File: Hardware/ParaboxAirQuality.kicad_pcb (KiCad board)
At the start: 2 copper layers, 25 parts, among them J1 USB_B_Mini, J2 Conn_01x03, J3 Conn_01x04, M1 CC2538MODULE, U1 ST1S10PHR, U2 M25PX32-VMW

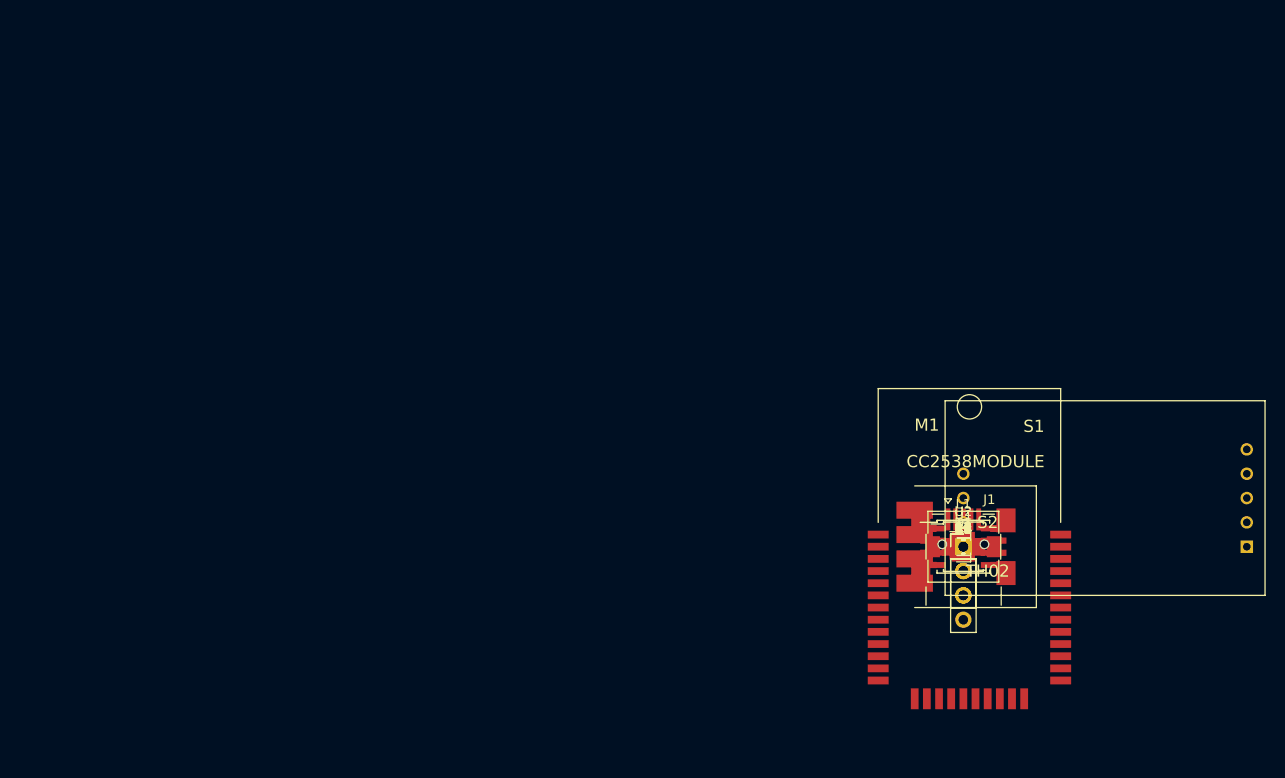
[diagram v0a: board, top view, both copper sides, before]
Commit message: Final release 1.0, add gerbers
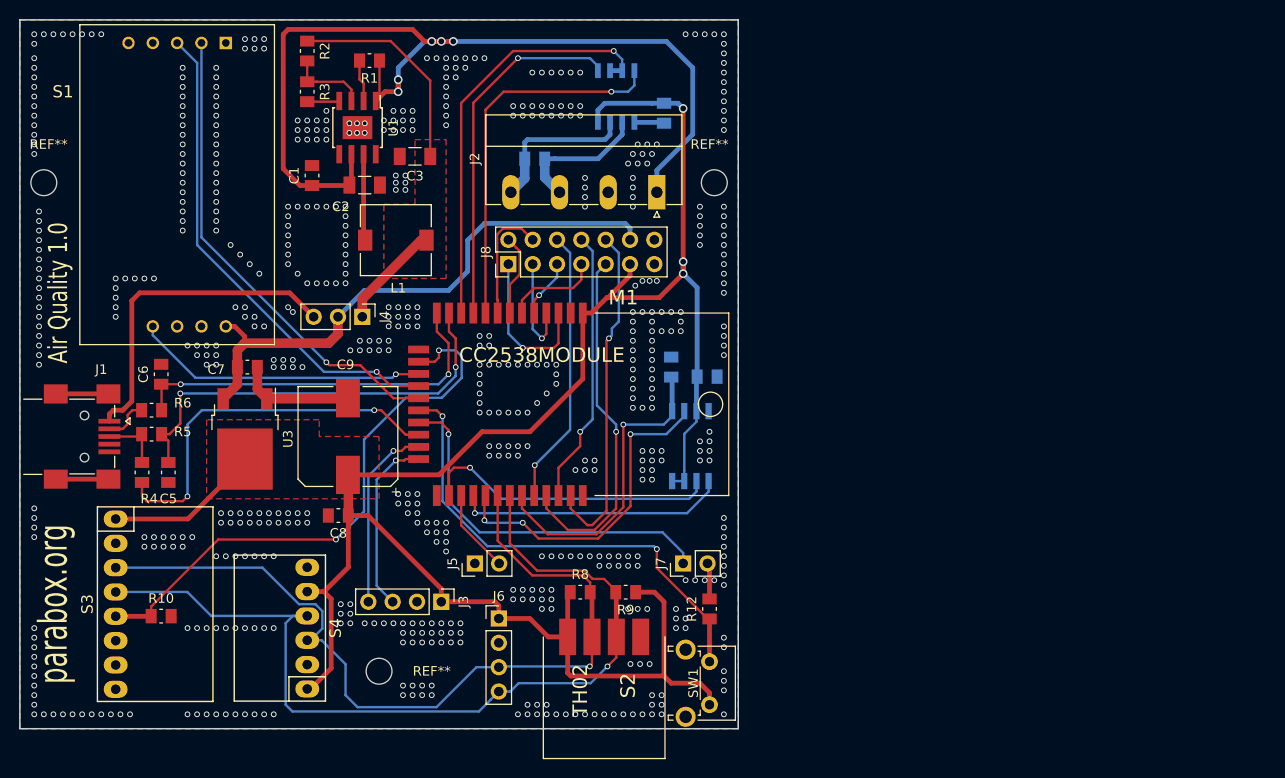
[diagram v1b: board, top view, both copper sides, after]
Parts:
- removed D1: BAT54C, Package_TO_SOT_SMD:SOT-23
- added C10: 0.1u, Capacitor_SMD:C_0805_2012Metric_Pad1.15x1.50mm_HandSolder, B.Cu at (117.2, 59.8)
- added C7: 0.1u, Capacitor_SMD:C_0805_2012Metric_Pad1.15x1.50mm_HandSolder, F.Cu at (73.8, 86.2)
- added C8: 0.1u, Capacitor_SMD:C_0805_2012Metric_Pad1.15x1.50mm_HandSolder, F.Cu at (83.2, 101.8)
- added C9: CP, Capacitor_SMD:CP_Elec_10x10, F.Cu at (84.2, 93.5)
- added J4: Conn_01x03, Connector_PinHeader_2.54mm:PinHeader_1x03_P2.54mm_Vertical, F.Cu at (85.8, 81.0)
- added J5: BOOT, Connector_PinHeader_2.54mm:PinHeader_1x02_P2.54mm_Vertical, F.Cu at (97.5, 106.8)
- added J6: I2C, Connector_PinHeader_2.54mm:PinHeader_1x04_P2.54mm_Vertical, F.Cu at (100.0, 112.5)
- added J7: BEEP, Connector_PinHeader_2.54mm:PinHeader_1x02_P2.54mm_Vertical, F.Cu at (119.2, 106.8)
- added J8: MISC, Connector_PinHeader_2.54mm:PinHeader_2x07_P2.54mm_Vertical, F.Cu at (101.0, 75.5)
- added R10: 10k, Resistor_SMD:R_0805_2012Metric_Pad1.15x1.50mm_HandSolder, F.Cu at (64.8, 112.2)
- added R11: 120, Resistor_SMD:R_0805_2012Metric_Pad1.15x1.50mm_HandSolder, B.Cu at (103.8, 64.5)
- added R12: 10k, Resistor_SMD:R_0805_2012Metric_Pad1.15x1.50mm_HandSolder, F.Cu at (122.0, 111.5)
- added REF**: MountingHole_2.7mm_M2.5, MountingHole:MountingHole_2.7mm_M2.5, F.Cu at (52.5, 67.0)
- added REF**: MountingHole_2.7mm_M2.5, MountingHole:MountingHole_2.7mm_M2.5, F.Cu at (122.5, 67.0)
- added REF**: MountingHole_2.7mm_M2.5, MountingHole:MountingHole_2.7mm_M2.5, F.Cu at (87.5, 118.0)
- added S3: CJMCU-811, Levap_Sensors:CJMCU-811, F.Cu at (60.0, 111.0)
- added S4: BMP280MOD, Levap_Sensors:BMP280MOD, F.Cu at (80.0, 113.5)
- added SW1: SW_Push, Button_Switch_THT:SW_Tactile_SPST_Angled_PTS645Vx83-2LFS, F.Cu at (122.0, 117.0)
- added U3: LM1117-3.3, Package_TO_SOT_SMD:TO-252-2, F.Cu at (73.5, 93.8)
- added U4: MAX3072E, Package_SO:SOIC-8_3.9x4.9mm_P1.27mm, B.Cu at (112.2, 58.0)
- C4, R7, U2: moved to B.Cu
- J2: value Conn_01x03 -> VIN; footprint Connector_PinHeader_2.54mm:PinHeader_1x03_P2.54mm_Vertical -> Connector_Phoenix_MC:PhoenixContact_MC_1,5_4-G-5.08_1x04_P5.08mm_Horizontal
- J3: value Conn_01x04 -> BOOT
- L1: footprint Inductors_SMD:L_7.3x7.3_H4.5 -> Inductor_SMD:L_7.3x7.3_H4.5
- R2: value 62.5k -> 105k
- moved J1 92.7 mm to (56.5, 93.5), turned to 270 degrees
- moved R4 86.1 mm to (62.8, 97.2), turned to 90 degrees
- moved R6 85.9 mm to (63.8, 90.8)
- moved R2 85.9 mm to (80.0, 53.2), turned to 270 degrees
- moved C6 85.7 mm to (64.8, 87.0), turned to 90 degrees
- moved R5 85.6 mm to (63.8, 93.2)
- moved C5 83.4 mm to (65.5, 97.2), turned to 270 degrees
- moved R3 83.4 mm to (80.0, 57.5), turned to 270 degrees
- moved S1 80.4 mm to (71.5, 82.0), turned to 90 degrees
- moved R1 80.1 mm to (86.5, 54.2), turned to 180 degrees
- moved C1 78.3 mm to (80.5, 66.2), turned to 90 degrees
- moved U1 76.9 mm to (85.2, 61.2), turned to 270 degrees
- moved C2 73.0 mm to (86.0, 67.2)
- moved C3 70.3 mm to (91.2, 64.2), turned to 180 degrees
- moved L1 67.3 mm to (89.2, 73.0)
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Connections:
- C1 pad 1: Vin -> VCC
- C2 pad 1: Vin -> VCC
- C3 pad 1: +3V3 -> /Vin_5V
- J2 pad 1: /EXT_Vin -> VCC
- J2 pad 2: Vin -> GND
- J2 pad 3: /USB_5V -> /RS485_A
- J3 pad 1: GND -> +3V3
- J3 pad 2: /UART0_BOOT_RX -> GND
- J3 pad 4: +3V3 -> /UART0_BOOT_RX
- L1 pad 2: +3V3 -> /Vin_5V
- M1 pad 10: Net-(M1-Pad10) -> /UART1_TX
- M1 pad 11: Net-(M1-Pad11) -> /RS485_RE-DE
- M1 pad 15: Net-(M1-Pad15) -> /CCS811_WAK
- M1 pad 19: /I2C_SDA -> /JOIN_BUT
- M1 pad 20: /I2C_SCK -> /BEEP
- M1 pad 29: Net-(M1-Pad29) -> /I2C_SCK
- M1 pad 3: Net-(M1-Pad3) -> /TMS
- M1 pad 30: Net-(M1-Pad30) -> /I2C_SDA
- M1 pad 32: Net-(M1-Pad32) -> /PD1
- M1 pad 33: Net-(M1-Pad33) -> /RESET
- M1 pad 34: Net-(M1-Pad34) -> /PD3
- M1 pad 35: Net-(M1-Pad35) -> /PD4
- M1 pad 4: Net-(M1-Pad4) -> /TCK
- M1 pad 5: Net-(M1-Pad5) -> /TDO/PB7
- M1 pad 6: Net-(M1-Pad6) -> /TDI/PB6
- M1 pad 7: Net-(M1-Pad7) -> /PB5
- M1 pad 8: Net-(M1-Pad8) -> /PB4
- M1 pad 9: Net-(M1-Pad9) -> /UART1_RX
- R1 pad 1: Vin -> VCC
- R2 pad 1: +3V3 -> /Vin_5V
- S1 pad 6: +3V3 -> +5V
- U1 pad 1: Vin -> VCC
- U1 pad 6: Vin -> VCC
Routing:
- net +3V3: track 0.00 -> 214.9 mm, vias 0 -> 3
- net VCC: track 0.00 -> 103.9 mm, vias 0 -> 5
- net /I2C_SDA: track 0.00 -> 94.4 mm, vias 0 -> 1
- net /I2C_SCK: track 0.00 -> 88.5 mm, vias 0 -> 1
- net +5V: track 0.00 -> 59.6 mm
- net /CCS811_WAK: track 0.00 -> 59.4 mm, vias 0 -> 2
- net /UART0_RX: track 0.00 -> 51.2 mm, vias 0 -> 1
- net /JOIN_BUT: track 0.00 -> 50.2 mm, vias 0 -> 2
- net /UART0_TX: track 0.00 -> 49.9 mm, vias 0 -> 1
- net /USB_P: track 0.00 -> 45.2 mm, vias 0 -> 2
- net /RS485_RE-DE: track 0.00 -> 43.8 mm, vias 0 -> 1
- net /USB_N: track 0.00 -> 40.1 mm, vias 0 -> 2
- net /USB_PULL: track 0.00 -> 39.9 mm, vias 0 -> 2
- net /UART1_RX: track 0.00 -> 39.4 mm, vias 0 -> 1
- net /BEEP: track 0.00 -> 38.7 mm, vias 0 -> 1
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- added copper zone on F.Cu, net +3V3
- added copper zone on F.Cu, net /Vin_5V
- added copper zone on B.Cu, net GND
- added copper zone on F.Cu, net GND
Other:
- board outline added: 75 x 74 mm
- board text added: "Air Quality 1.0"
- board text added: "parabox.org"
